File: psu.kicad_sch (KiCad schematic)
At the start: 29 parts, among them U14 TPS563201DDCR, U15 LM1117-ADJ, U16 LM1117-ADJ

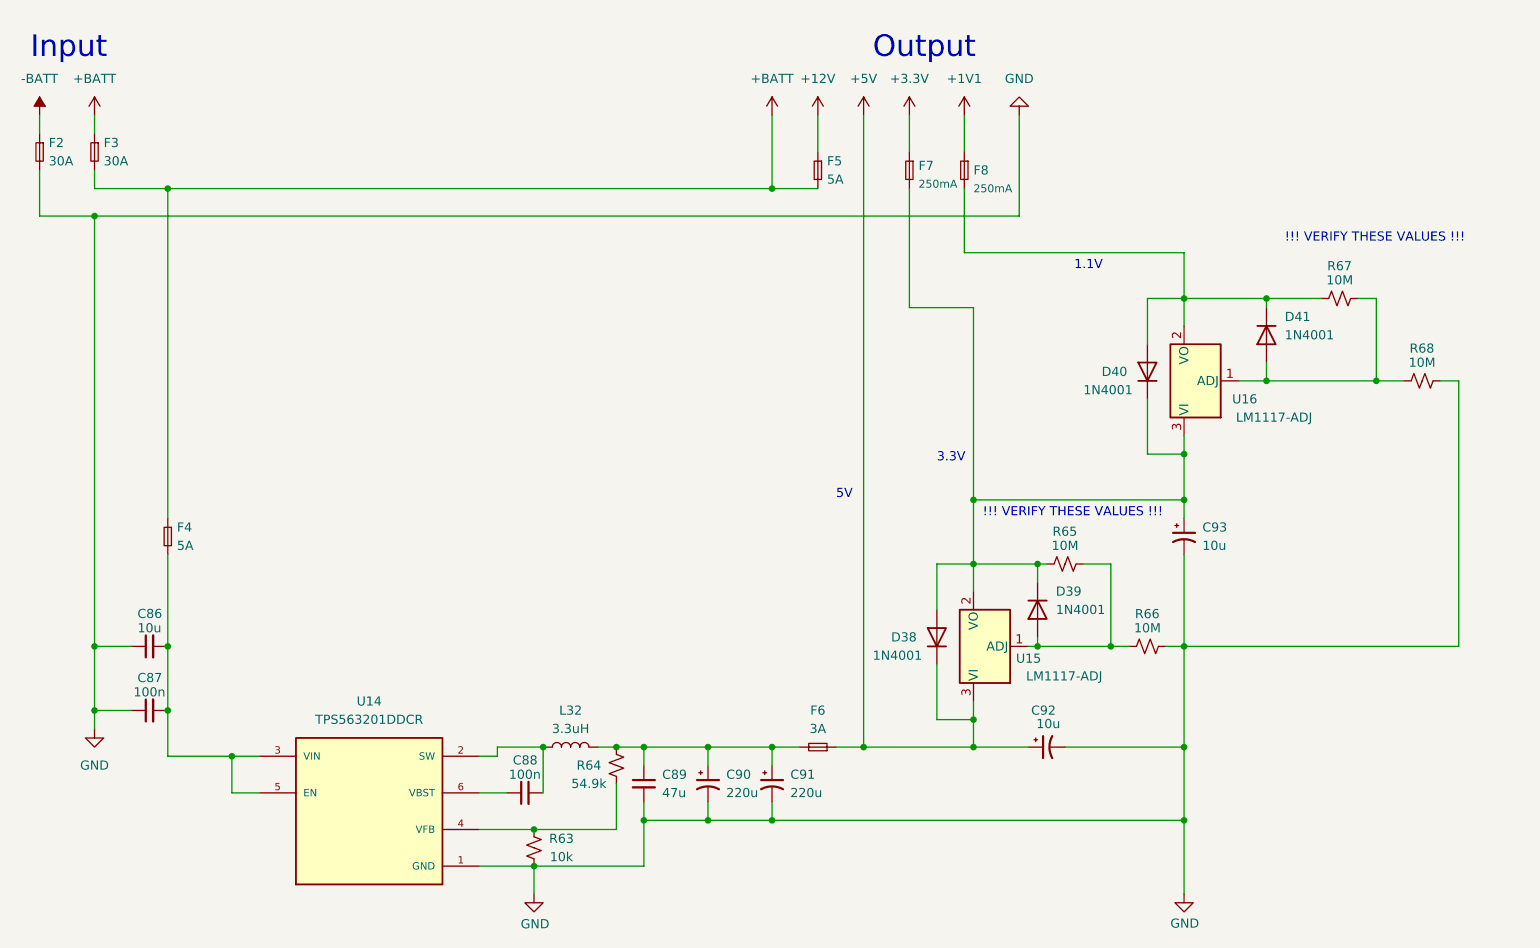
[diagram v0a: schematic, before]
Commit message: cleanup of schematic and some initial firmware works...
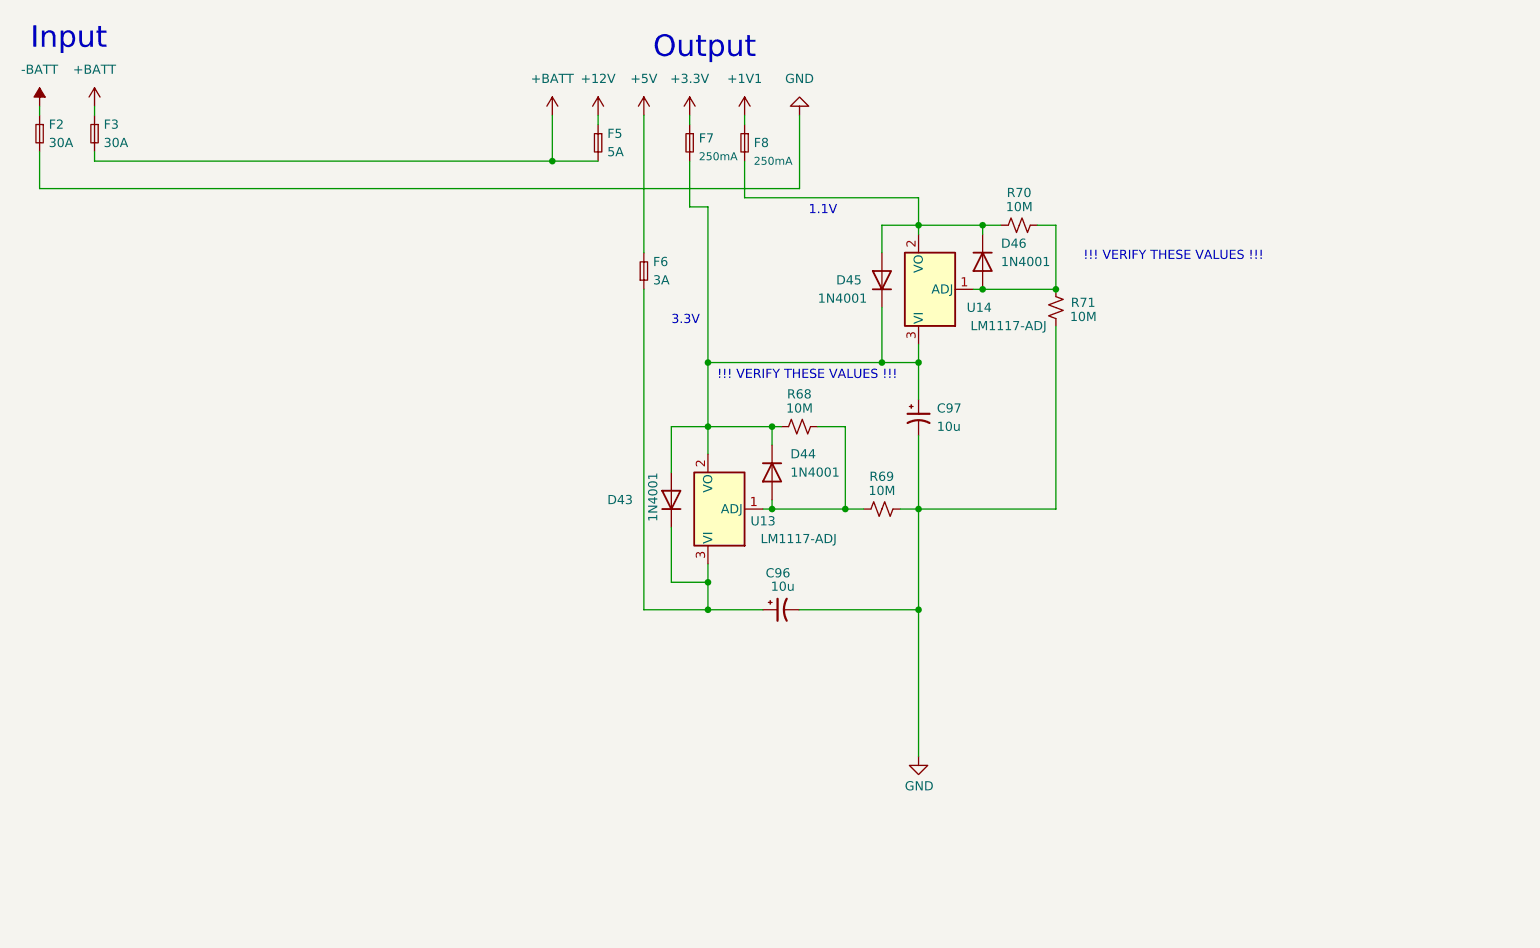
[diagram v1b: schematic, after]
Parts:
- removed C86: 10u, Capacitor_THT:C_Disc_D4.7mm_W2.5mm_P5.00mm, symbol Device:C_Small
- removed C87, C88: 100n, Capacitor_THT:C_Disc_D4.7mm_W2.5mm_P5.00mm, symbol Device:C_Small
- removed C89: 47u, Capacitor_THT:C_Disc_D4.7mm_W2.5mm_P5.00mm, symbol Device:C_Small
- removed C90, C91: 220u, Capacitor_THT:CP_Radial_D4.0mm_P2.00mm, symbol Device:C_Polarized_Small_US
- removed C92, C93: 10u, Capacitor_THT:CP_Radial_D4.0mm_P2.00mm, symbol Device:C_Polarized_Small_US
- removed D38, D39, D40, D41: 1N4001, Diode_THT:D_DO-41_SOD81_P10.16mm_Horizontal, symbol Diode:1N4001
- removed F4: 5A, Fuse:Fuseholder_Blade_Mini_Keystone_3568, symbol Device:Fuse_Small
- removed L32: 3.3uH, symbol Device:L
- removed R63: 10k, Resistor_THT:R_Axial_DIN0207_L6.3mm_D2.5mm_P2.54mm_Vertical, symbol Device:R_Small_US
- removed R64: 54.9k, Resistor_THT:R_Axial_DIN0207_L6.3mm_D2.5mm_P2.54mm_Vertical, symbol Device:R_Small_US
- removed R65, R66, R67: 10M, Resistor_THT:R_Axial_DIN0207_L6.3mm_D2.5mm_P2.54mm_Vertical, symbol Device:R_Small_US
- removed U14: TPS563201DDCR, SOT95P280X110-6N, symbol TPS563201DDCR:TPS563201DDCR
- removed U15, U16: LM1117-ADJ, symbol Regulator_Linear:LM1117-ADJ
- added C96, C97: 10u, Capacitor_THT:CP_Radial_D4.0mm_P2.00mm, symbol Device:C_Polarized_Small_US
- added D43, D44, D45, D46: 1N4001, Diode_THT:D_DO-41_SOD81_P10.16mm_Horizontal, symbol Diode:1N4001
- added R69, R70, R71: 10M, Resistor_THT:R_Axial_DIN0207_L6.3mm_D2.5mm_P2.54mm_Vertical, symbol Device:R_Small_US
- added U13, U14: LM1117-ADJ, symbol Regulator_Linear:LM1117-ADJ
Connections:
- net +5V: now also F6.2; no longer F6.1
- net GND: now also C96.2, C97.2, R69.2, R71.2; no longer R68.2
- net at F8.2: now also D45.2 (A), D46.1 (K), R70.1, U14.2 (VO)
- net at F7.2: now also R68.1, C97.1, D43.2 (A), D44.1 (K), D45.1 (K), U13.2 (VO), U14.3 (VI)
- new net: C96.1, D43.1 (K), F6.1, U13.3 (VI)
- new net: D46.2 (A), R70.2, R71.1, U14.1 (ADJ)
- new net: D44.2 (A), R68.2, R69.1, U13.1 (ADJ)
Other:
- note removed: "5V"
